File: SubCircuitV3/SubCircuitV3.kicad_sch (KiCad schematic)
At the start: 23 parts, among them J1 JTAG, J10 ESC_POWER, J11 ESC_POWER, J12 ESC_POWER, J13 ESC_POWER, J14 FEMALE XT-60, J15 ESC PWM, J16 3S, J2 ESC PWM, J3 ESC PWM, J4 ESC PWM, J5 ESC PWM, J6 ESC PWM, J7 5S, J8 ESC_POWER, J9 ESC_POWER, K1 G5Q-1A

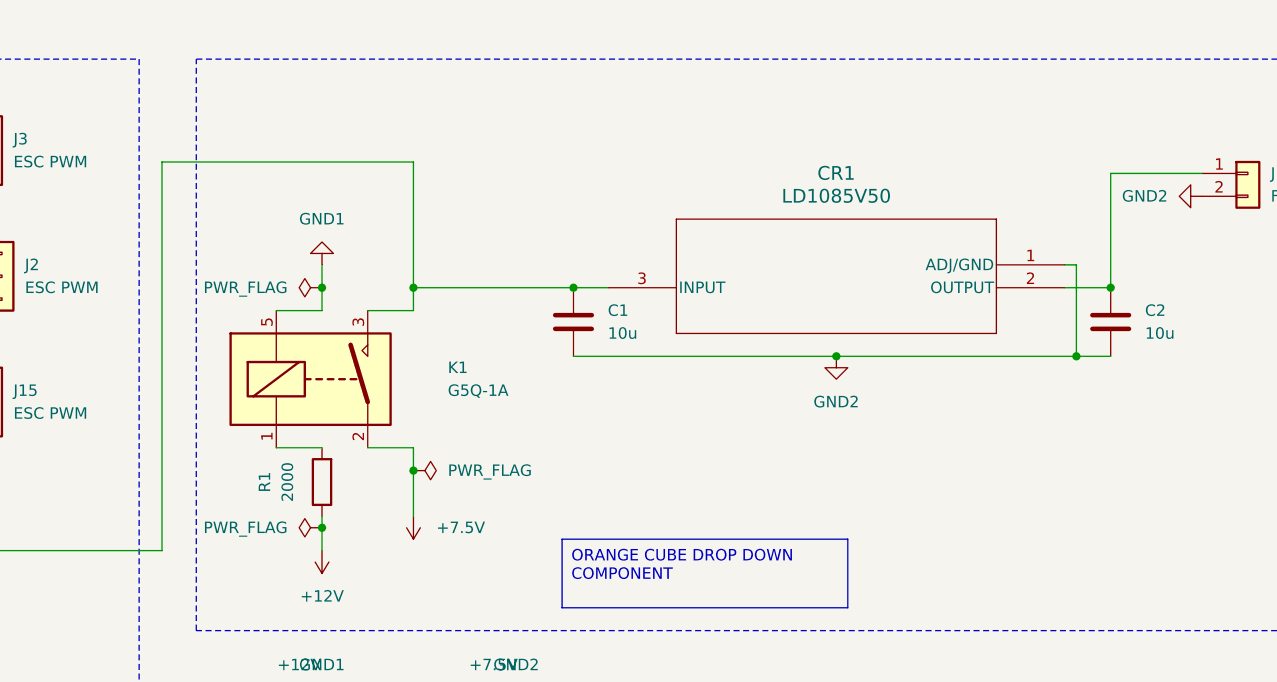
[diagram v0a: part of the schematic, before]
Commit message: Finalized V3 Board
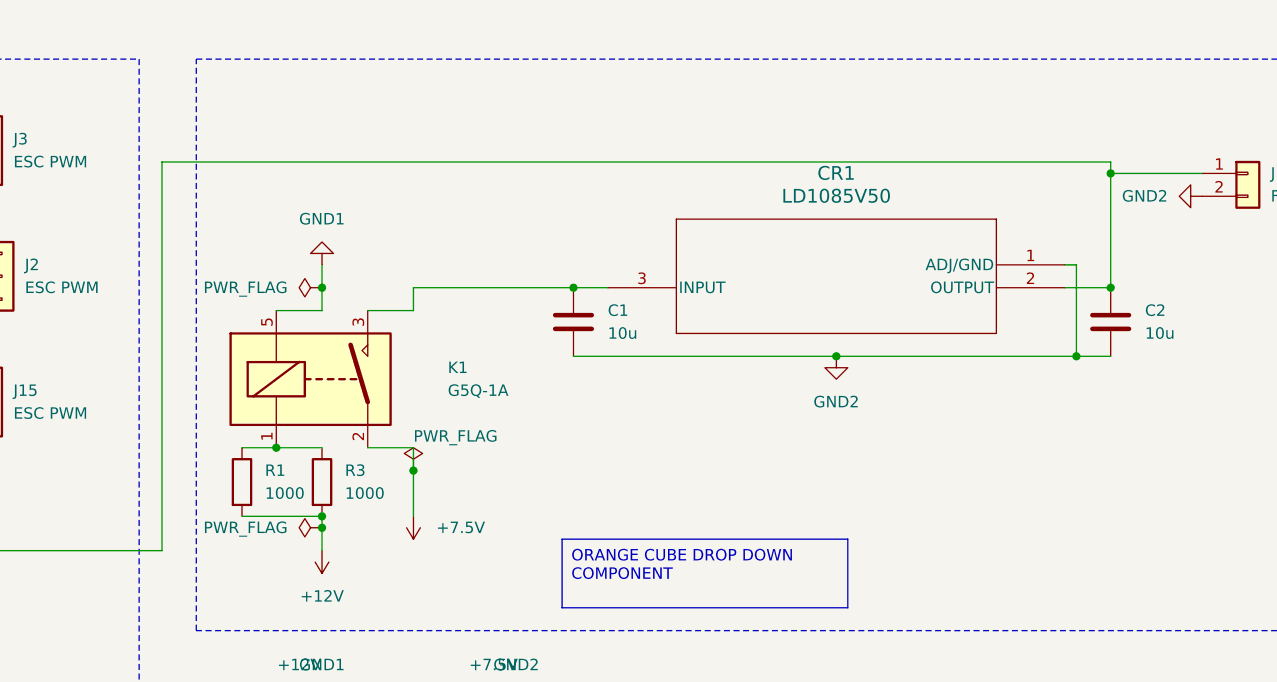
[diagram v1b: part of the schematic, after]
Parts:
- added R3: 1000, Resistor_THT:R_Axial_DIN0207_L6.3mm_D2.5mm_P10.16mm_Horizontal, symbol Device:R
- R1: value 2000 -> 1000
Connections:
- net +12V: now also R1.2, R3.2; no longer R1.1
- net at K1.1: now also R1.1, R3.1; no longer R1.2
- net at C1.1, CR1.3 (INPUT), K1.3: no longer J1.14 (Pin_14)
- net at C2.1, CR1.2 (OUTPUT), J14.1 (Pin_1): now also J1.14 (Pin_14)
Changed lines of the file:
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@@
   (junction (at 247.65 95.25) (diameter 0) (color 0 0 0 0)
   )
-  (junction (at 170.18 95.25) (diameter 0) (color 0 0 0 0)
-  )
   (junction (at 104.14 137.16) (diameter 0) (color 0 0 0 0)
   )
@@
   (junction (at 170.18 115.57) (diameter 0) (color 0 0 0 0)
   )
+  (junction (at 247.65 82.55) (diameter 0) (color 0 0 0 0)
+  )
   (junction (at 243.84 102.87) (diameter 0) (color 0 0 0 0)
+  )
+  (junction (at 160.02 120.65) (diameter 0) (color 0 0 0 0)
+  )
+  (junction (at 154.94 113.03) (diameter 0) (color 0 0 0 0)
   )
   (junction (at 187.96 95.25) (diameter 0) (color 0 0 0 0)
@@
   (no_connect (at 96.52 107.95))
   (no_connect (at 97.79 93.98))
+  (wire (pts (xy 151.13 113.03) (xy 154.94 113.03))
+    (stroke (width 0) (type default))
+  )
   (wire (pts (xy 109.22 77.47) (xy 109.22 124.46))
     (stroke (width 0) (type default))
@@
     (stroke (width 0) (type default))
   )
-  (wire (pts (xy 160.02 113.03) (xy 154.94 113.03))
-    (stroke (width 0) (type default))
-  )
   (wire (pts (xy 116.84 124.46) (xy 142.24 124.46))
     (stroke (width 0) (type default))
@@
     (stroke (width 0) (type default))
   )
-  (wire (pts (xy 170.18 81.28) (xy 170.18 95.25))
-    (stroke (width 0) (type default))
-  )
   (wire (pts (xy 111.76 91.44) (xy 111.76 124.46))
     (stroke (width 0) (type default))
@@
     (stroke (width 0) (type default))
   )
-  (wire (pts (xy 142.24 81.28) (xy 170.18 81.28))
+  (wire (pts (xy 142.24 81.28) (xy 247.65 81.28))
     (stroke (width 0) (type default))
   )
@@
     (stroke (width 0) (type default))
   )
+  (wire (pts (xy 154.94 113.03) (xy 160.02 113.03))
+    (stroke (width 0) (type default))
+  )
   (wire (pts (xy 242.57 95.25) (xy 247.65 95.25))
     (stroke (width 0) (type default))
@@
     (stroke (width 0) (type default))
   )
+  (wire (pts (xy 247.65 81.28) (xy 247.65 82.55))
+    (stroke (width 0) (type default))
+  )
   (wire (pts (xy 97.79 91.44) (xy 104.14 91.44))
     (stroke (width 0) (type default))
@@
   )
   (wire (pts (xy 106.68 137.16) (xy 107.95 137.16))
+    (stroke (width 0) (type default))
+  )
+  (wire (pts (xy 151.13 120.65) (xy 160.02 120.65))
     (stroke (width 0) (type default))
   )
@@
     (effects (font (size 1.27 1.27)) (justify left top))
   )
-  (symbol (lib_id "power:PWR_FLAG") (at 170.18 115.57 270) (unit 1)
-    (in_bom yes) (on_board yes) (dnp no) (fields_autoplaced)
-    (property "Reference" "#FLG02" (at 172.085 115.57 0)
-      (effects (font (size 1.27 1.27)) hide)
-    )
-    (property "Value" "PWR_FLAG" (at 173.99 115.57 90)
+  (symbol (lib_id "power:PWR_FLAG") (at 170.18 115.57 0) (unit 1)
+    (in_bom yes) (on_board yes) (dnp no)
+    (property "Reference" "#FLG02" (at 170.18 113.665 0)
+      (effects (font (size 1.27 1.27)) hide)
+    )
+    (property "Value" "PWR_FLAG" (at 170.18 111.76 0)
       (effects (font (size 1.27 1.27)) (justify left))
     )
@@
     )
   )
-  (symbol (lib_id "Device:R") (at 160.02 116.84 180) (unit 1)
+  (symbol (lib_id "power:+7.5V") (at 170.18 120.65 180) (unit 1)
     (in_bom yes) (on_board yes) (dnp no)
-    (property "Reference" "R1" (at 153.67 116.84 90)
-      (effects (font (size 1.27 1.27)))
-    )
-    (property "Value" "2000" (at 156.21 116.84 90)
-      (effects (font (size 1.27 1.27)))
-    )
-    (property "Footprint" "Resistor_THT:R_Axial_DIN0207_L6.3mm_D2.5mm_P10.16mm_Horizontal" (at 161.798 116.84 90)
-      (effects (font (size 1.27 1.27)) hide)
-    )
-    (property "Datasheet" "~" (at 160.02 116.84 0)
-      (effects (font (size 1.27 1.27)) hide)
-    )
-    (pin "1")
-    (pin "2")
-    (instances
-      (project "SubCircuitV3"
-        (path "/364d75d3-77e7-4f3e-a207-f79712f2b174"
-          (reference "R1") (unit 1)
-        )
-      )
-    )
-  )
-  (symbol (lib_id "power:+7.5V") (at 170.18 120.65 180) (unit 1)
-    (in_bom yes) (on_board yes) (dnp no) (fields_autoplaced)
     (property "Reference" "#PWR010" (at 170.18 116.84 0)
       (effects (font (size 1.27 1.27)) hide)
@@
         (path "/364d75d3-77e7-4f3e-a207-f79712f2b174"
           (reference "#PWR09") (unit 1)
+        )
+      )
+    )
+  )
+  (symbol (lib_id "Device:R") (at 160.02 116.84 0) (unit 1)
+    (in_bom yes) (on_board yes) (dnp no) (fields_autoplaced)
+    (property "Reference" "R3" (at 162.56 115.57 0)
+      (effects (font (size 1.27 1.27)) (justify left))
+    )
+    (property "Value" "1000" (at 162.56 118.11 0)
+      (effects (font (size 1.27 1.27)) (justify left))
+    )
+    (property "Footprint" "Resistor_THT:R_Axial_DIN0207_L6.3mm_D2.5mm_P10.16mm_Horizontal" (at 158.242 116.84 90)
+      (effects (font (size 1.27 1.27)) hide)
+    )
+    (property "Datasheet" "~" (at 160.02 116.84 0)
+      (effects (font (size 1.27 1.27)) hide)
+    )
+    (pin "1")
+    (pin "2")
+    (instances
+      (project "SubCircuitV3"
+        (path "/364d75d3-77e7-4f3e-a207-f79712f2b174"
+          (reference "R3") (unit 1)
         )
       )
@@
         )
       )
+    )
+  )
+  (symbol (lib_id "Device:R") (at 151.13 116.84 0) (unit 1)
+    (in_bom yes) (on_board yes) (dnp no) (fields_autoplaced)
+    (property "Reference" "R1" (at 153.67 115.57 0)
+      (effects (font (size 1.27 1.27)) (justify left))
+    )
+    (property "Value" "1000" (at 153.67 118.11 0)
+      (effects (font (size 1.27 1.27)) (justify left))
+    )
+    (property "Footprint" "Resistor_THT:R_Axial_DIN0207_L6.3mm_D2.5mm_P10.16mm_Horizontal" (at 149.352 116.84 90)
+      (effects (font (size 1.27 1.27)) hide)
+    )
+    (property "Datasheet" "~" (at 151.13 116.84 0)
+      (effects (font (size 1.27 1.27)) hide)
+    )
+    (pin "1")
+    (pin "2")
+    (instances
+      (project "SubCircuitV3"
+        (path "/364d75d3-77e7-4f3e-a207-f79712f2b174"
+          (reference "R1") (unit 1)
+        )
+      )
